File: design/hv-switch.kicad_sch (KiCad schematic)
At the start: 29 parts, among them Q3 GAN080-650EBE, U7 MAX22702EASA+

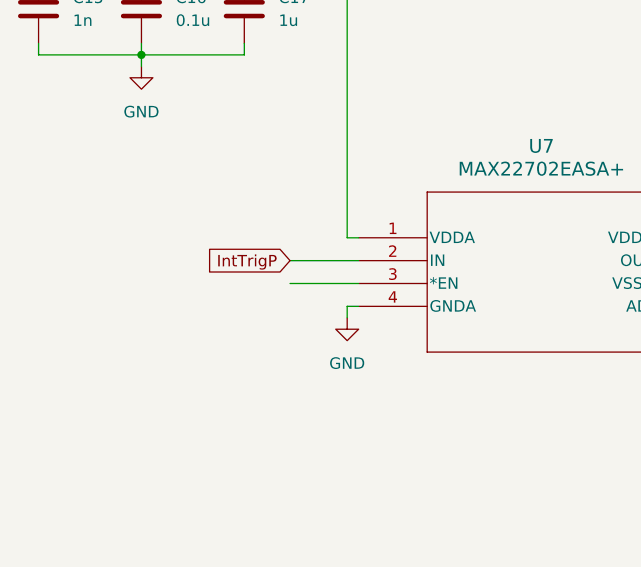
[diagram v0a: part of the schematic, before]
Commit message: _
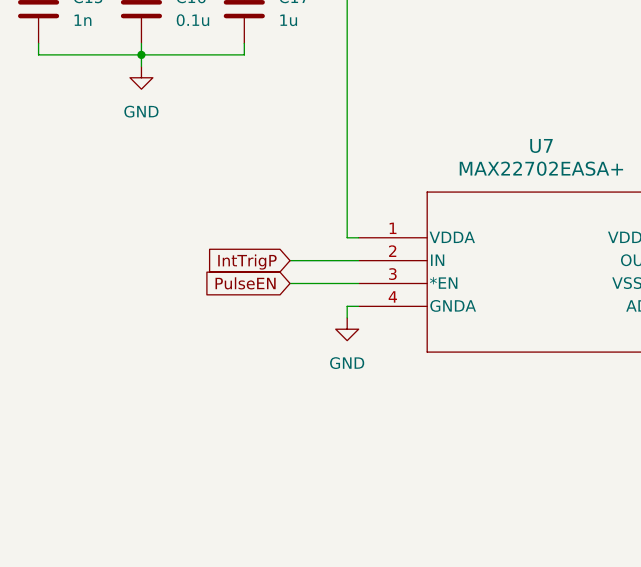
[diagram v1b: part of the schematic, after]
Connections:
- net PulseEN: now reaches U7.3 (*EN)
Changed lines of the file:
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@@
+		)
+	)
+	(global_label "PulseEN"
+		(shape input)
+		(at 62.23 78.74 180)
+		(fields_autoplaced yes)
+		(effects
+			(font
+				(size 1.27 1.27)
+			)
+			(justify right)
+		)
+		(property "Intersheetrefs" "${INTERSHEET_REFS}"
+			(at 51.5644 78.74 0)
+			(effects
+				(font
+					(size 1.27 1.27)
+				)
+				(justify right)
+				(hide yes)
+			)
 		)
 	)
